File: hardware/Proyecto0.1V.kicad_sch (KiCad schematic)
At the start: 0 parts

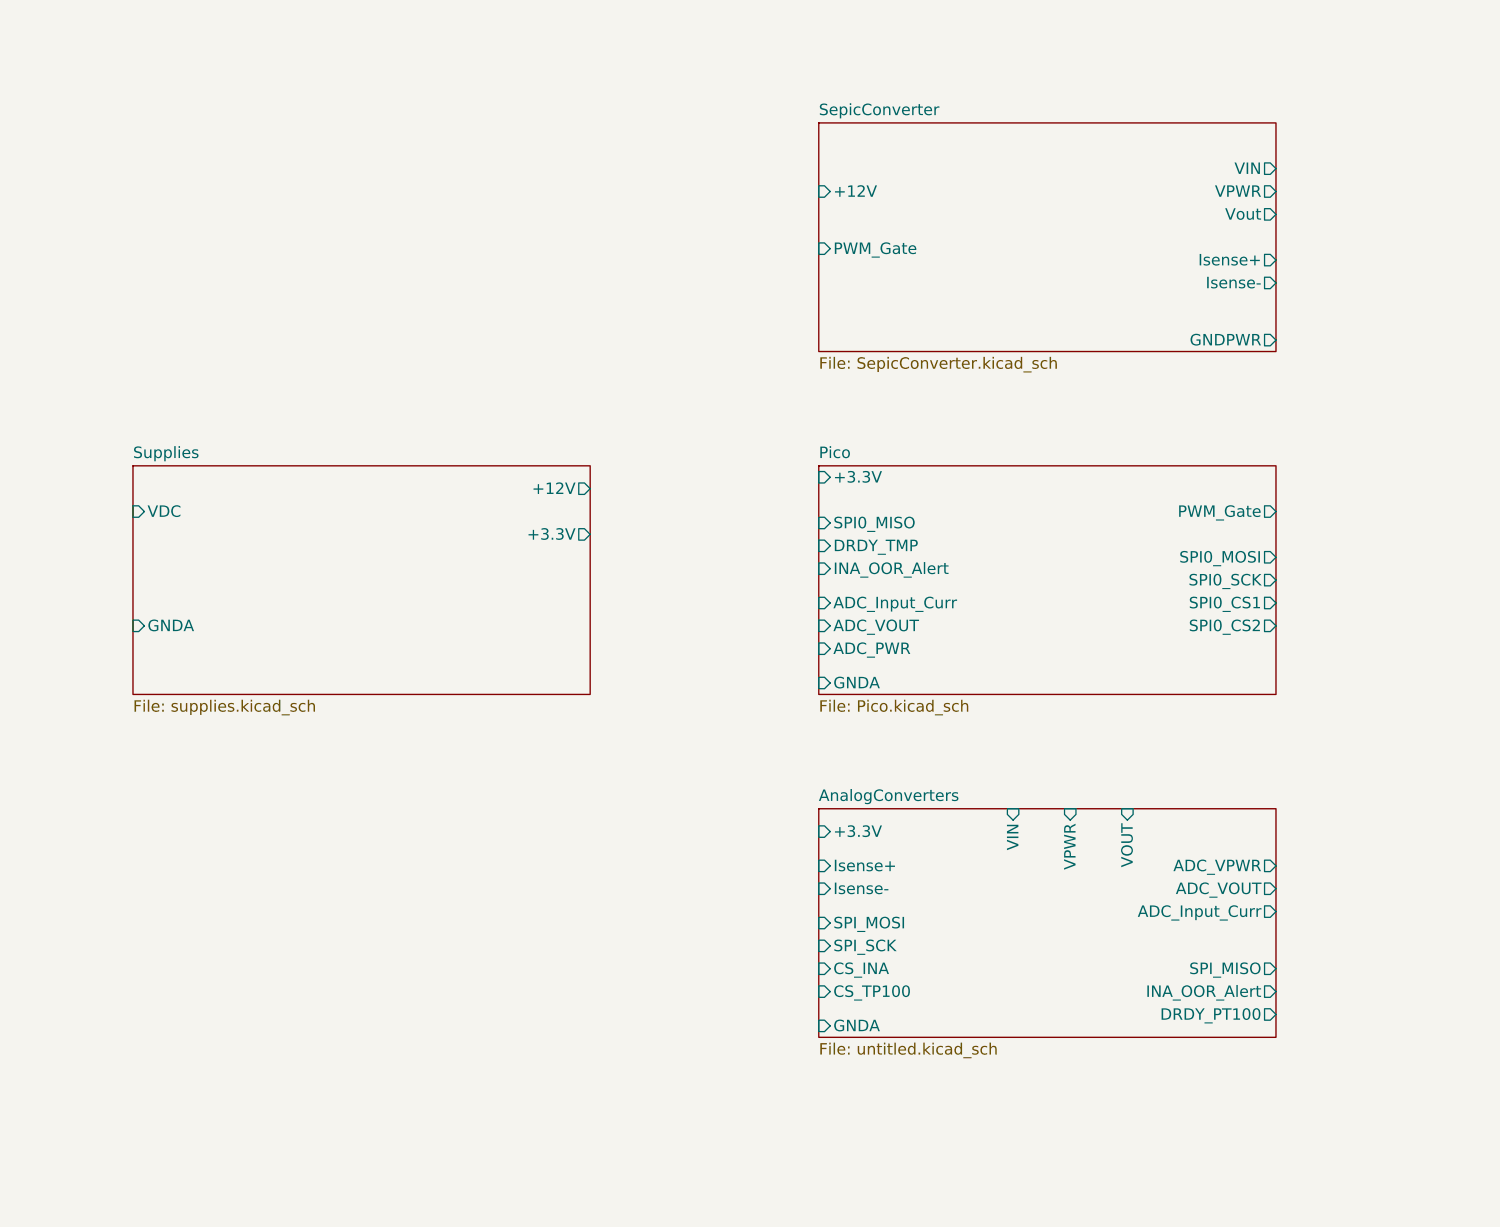
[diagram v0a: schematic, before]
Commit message: HW: Sch done. PCB WIP
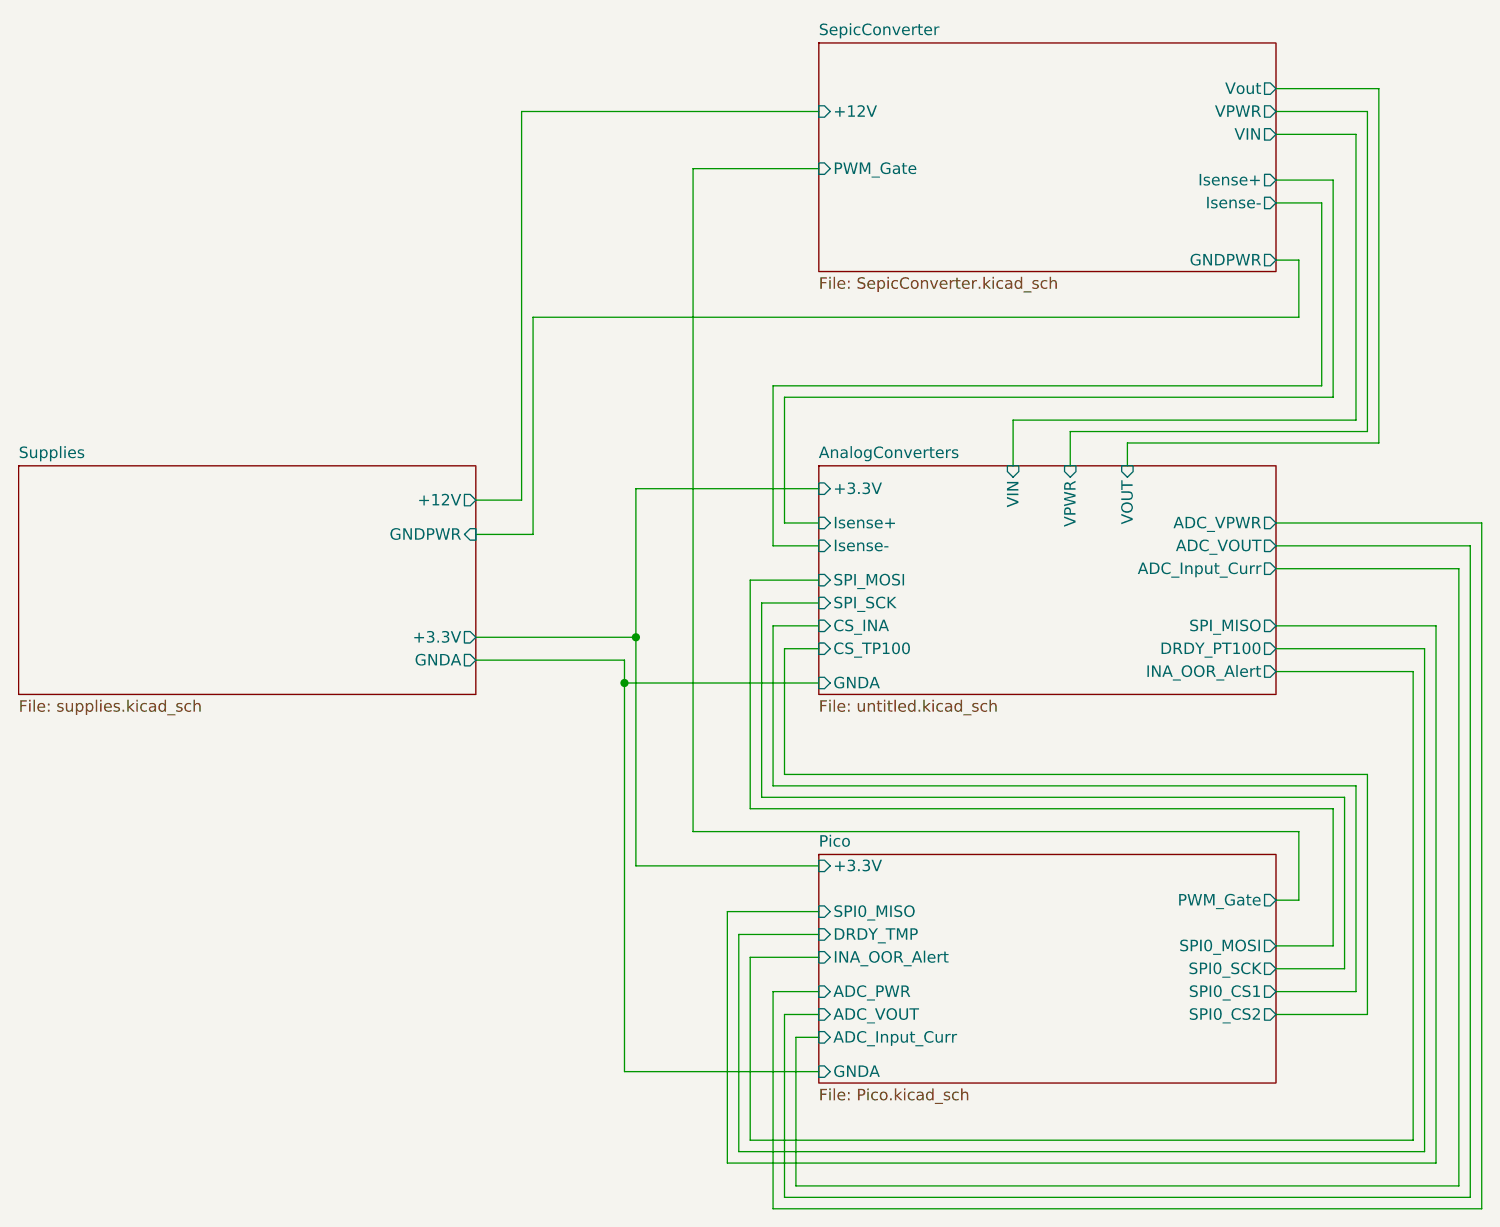
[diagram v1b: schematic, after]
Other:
- sheet Supplies ports: added GNDPWR; removed VDC
